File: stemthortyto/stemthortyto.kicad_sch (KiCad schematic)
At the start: 65 parts, among them IC1 E22-900M22S, J1 Jack-DC, Q1 BCV29, U1 LT1585-3.3, U2 ADXL343, U3 RK3588S, U4 K4UCE3Q4AB-MGCL, U5 FEMDRW032G-88A19

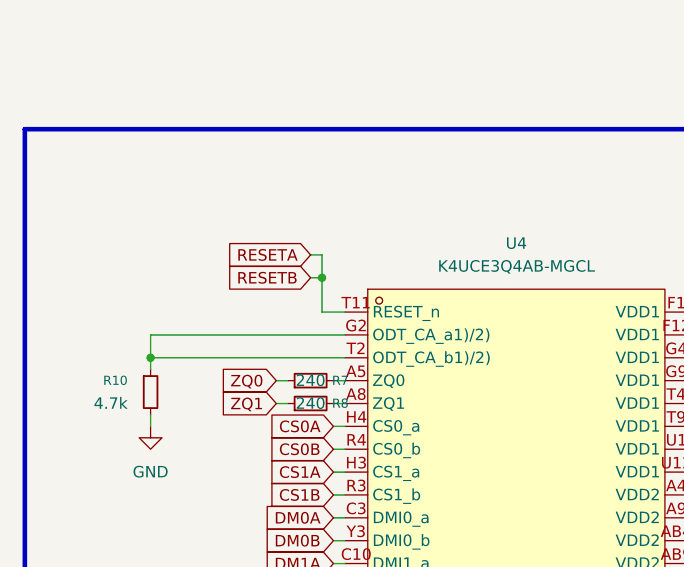
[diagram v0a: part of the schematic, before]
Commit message: Add files via upload
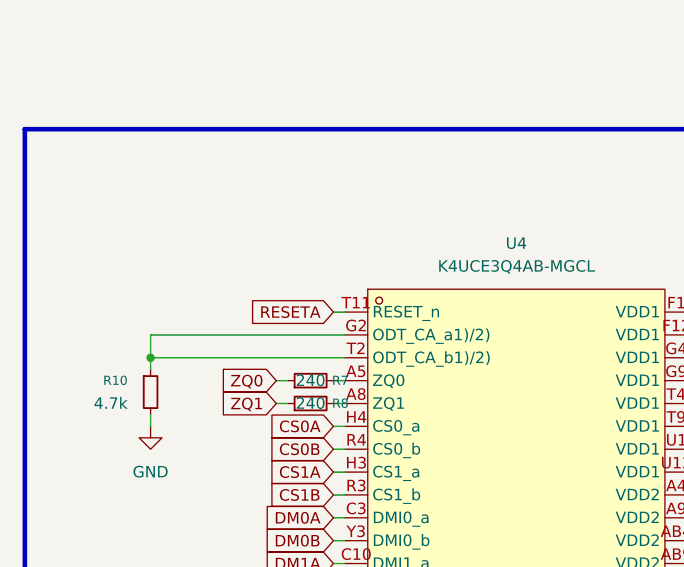
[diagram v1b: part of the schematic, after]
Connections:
- net RESETA: no longer U3.P1 (DDR_CH0_RESET_B)
- new net RESETB: U3.P1 (DDR_CH0_RESET_B)
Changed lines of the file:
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@@
 	)
 	(junction
-		(at 46.99 429.26)
-		(diameter 0)
-		(color 0 0 0 0)
-	)
-	(junction
 		(at 88.9 648.97)
 		(diameter 0)
@@
 	(wire
 		(pts
-			(xy 46.99 429.26) (xy 46.99 433.07)
-		)
-		(stroke
-			(width 0)
-			(type default)
-		)
-	)
-	(wire
-		(pts
 			(xy 48.26 636.27) (xy 49.53 636.27)
 		)
@@
 	(wire
 		(pts
-			(xy 49.53 433.07) (xy 46.99 433.07)
+			(xy 49.53 433.07) (xy 48.26 433.07)
 		)
 		(stroke
@@
 	(wire
 		(pts
-			(xy 45.72 426.72) (xy 46.99 426.72)
-		)
-		(stroke
-			(width 0)
-			(type default)
-		)
-	)
-	(wire
-		(pts
 			(xy 48.26 610.87) (xy 49.53 610.87)
 		)
@@
 	(wire
 		(pts
-			(xy 45.72 429.26) (xy 46.99 429.26)
-		)
-		(stroke
-			(width 0)
-			(type default)
-		)
-	)
-	(wire
-		(pts
 			(xy 123.19 190.5) (xy 125.73 190.5)
 		)
@@
 	(wire
 		(pts
-			(xy 46.99 426.72) (xy 46.99 429.26)
-		)
-		(stroke
-			(width 0)
-			(type default)
-		)
-	)
-	(wire
-		(pts
 			(xy 96.52 455.93) (xy 106.68 455.93)
 		)
@@
 	(global_label "RESETA"
 		(shape input)
-		(at 45.72 426.72 180)
+		(at 48.26 433.07 180)
 		(fields_autoplaced yes)
 		(effects
@@
 		)
 		(property "Intersheetrefs" "${INTERSHEET_REFS}"
-			(at 35.9011 426.72 0)
+			(at 38.4411 433.07 0)
 			(hide yes)
 			(show_name no)
@@
 			(hide yes)
 			(show_name no)
-			(do_not_autoplace no)
-			(effects
-				(font
-					(size 1.27 1.27)
-				)
-				(justify right)
-			)
-		)
-	)
-	(global_label "RESETB"
-		(shape input)
-		(at 45.72 429.26 180)
-		(fields_autoplaced yes)
-		(effects
-			(font
-				(size 1.27 1.27)
-			)
-			(justify right)
-		)
-		(property "Intersheetrefs" "${INTERSHEET_REFS}"
-			(at 35.7197 429.26 0)
-			(hide yes)
-			(show_name no)
